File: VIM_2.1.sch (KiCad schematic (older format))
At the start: 13 parts, among them J1 BARREL_JACK, J2 Sliding switch, U14 LD1117, U8 lm2596 - 5v, U9 LD1117S33CTR

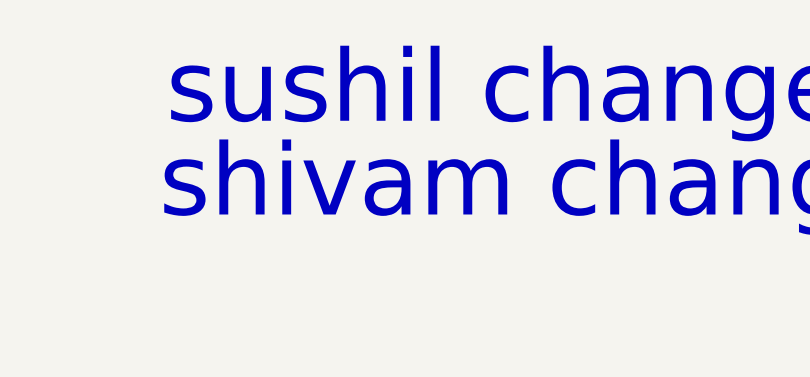
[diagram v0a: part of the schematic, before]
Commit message: changes to b
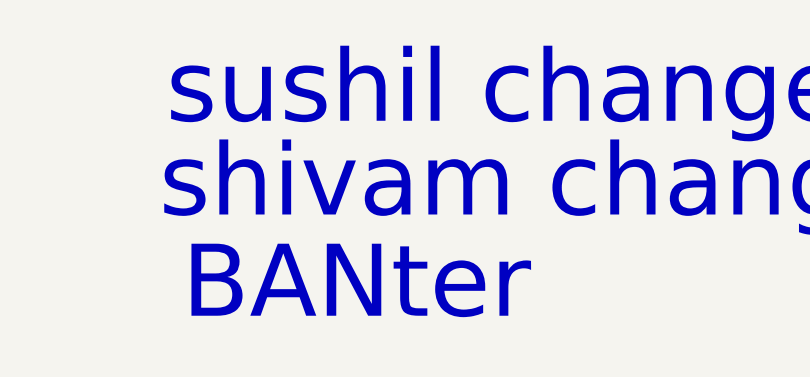
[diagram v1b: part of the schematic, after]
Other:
- note added: "BANter\n\n"
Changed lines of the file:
@@
 LIBS:mpu
 LIBS:68 PIN
-LIBS:reugulators
 LIBS:simcard
 LIBS:j502
@@
 Text Notes 3550 6300 0    315  ~ 0
 shivam changes\n
+Text Notes 3650 7250 0    315  ~ 0
+BANter\n\n
 $EndSCHEMATC

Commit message: Revert "changes to b"
This reverts commit 29845ce44828af67f545c5cae162d888299830da.
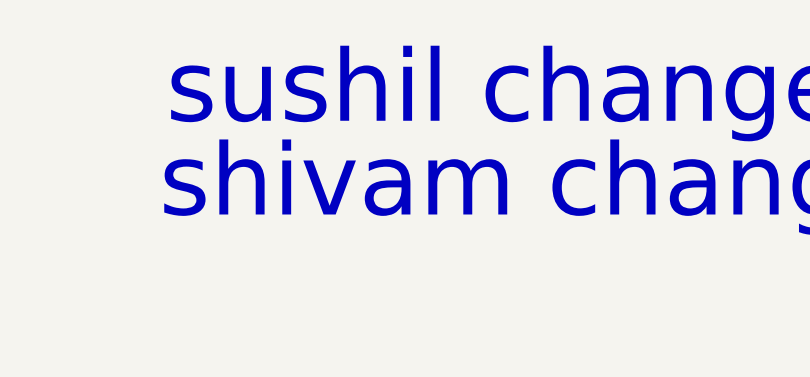
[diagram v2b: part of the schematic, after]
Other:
- note removed: "BANter\n\n"
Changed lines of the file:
@@
 LIBS:mpu
 LIBS:68 PIN
+LIBS:reugulators
 LIBS:simcard
 LIBS:j502
@@
 Text Notes 3550 6300 0    315  ~ 0
 shivam changes\n
-Text Notes 3650 7250 0    315  ~ 0
-BANter\n\n
 $EndSCHEMATC
